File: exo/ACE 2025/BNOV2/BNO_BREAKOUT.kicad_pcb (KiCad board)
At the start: 2 copper layers, 42 x 61.1 mm, 21 parts, among them M3 MountingHole_3.2mm_M3, U2 PCA9615DPZ, U3 AP7361C-33E

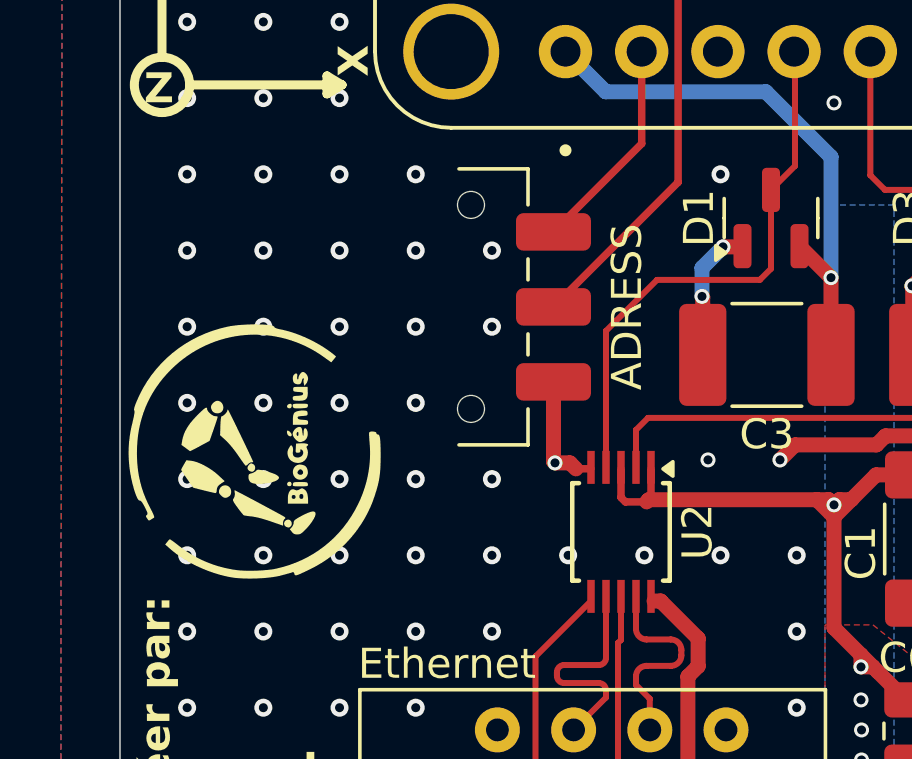
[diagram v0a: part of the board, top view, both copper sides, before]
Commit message: Push BNO et Moustache Gerber
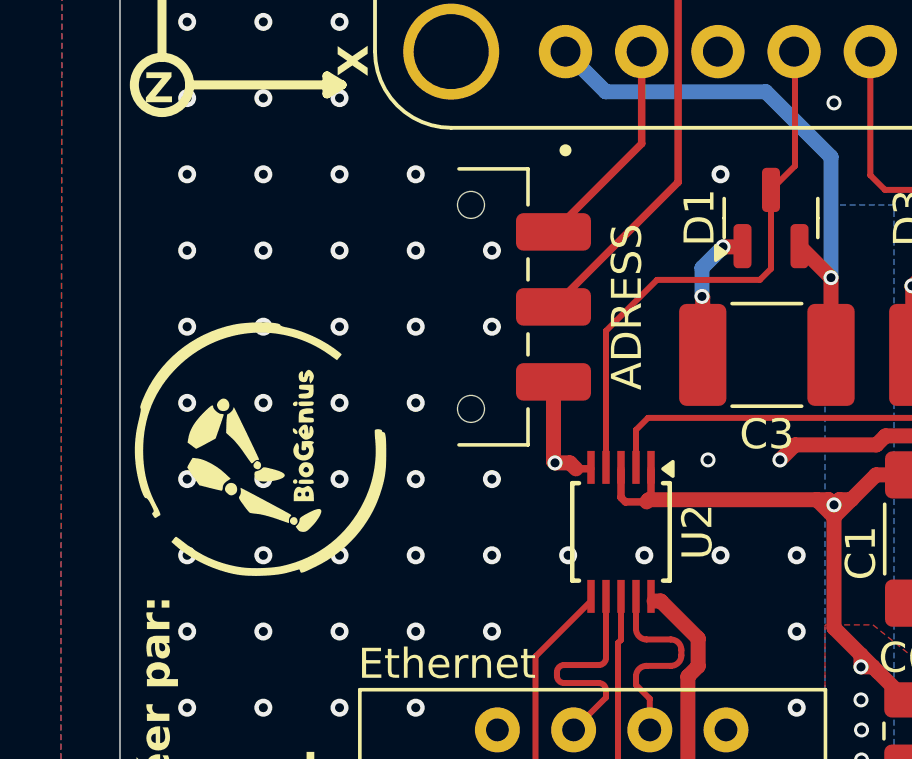
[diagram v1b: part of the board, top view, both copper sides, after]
